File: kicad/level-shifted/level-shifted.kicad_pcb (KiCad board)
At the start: 4 copper layers, 53.5 x 76 mm, 15 parts, among them J101 PAL-1 Expansion Connector, SW101 PICO RESET, U101 74LVC245, U102 74LVC245, U103 Pico, U104 74LVC245, U105 74LVC245

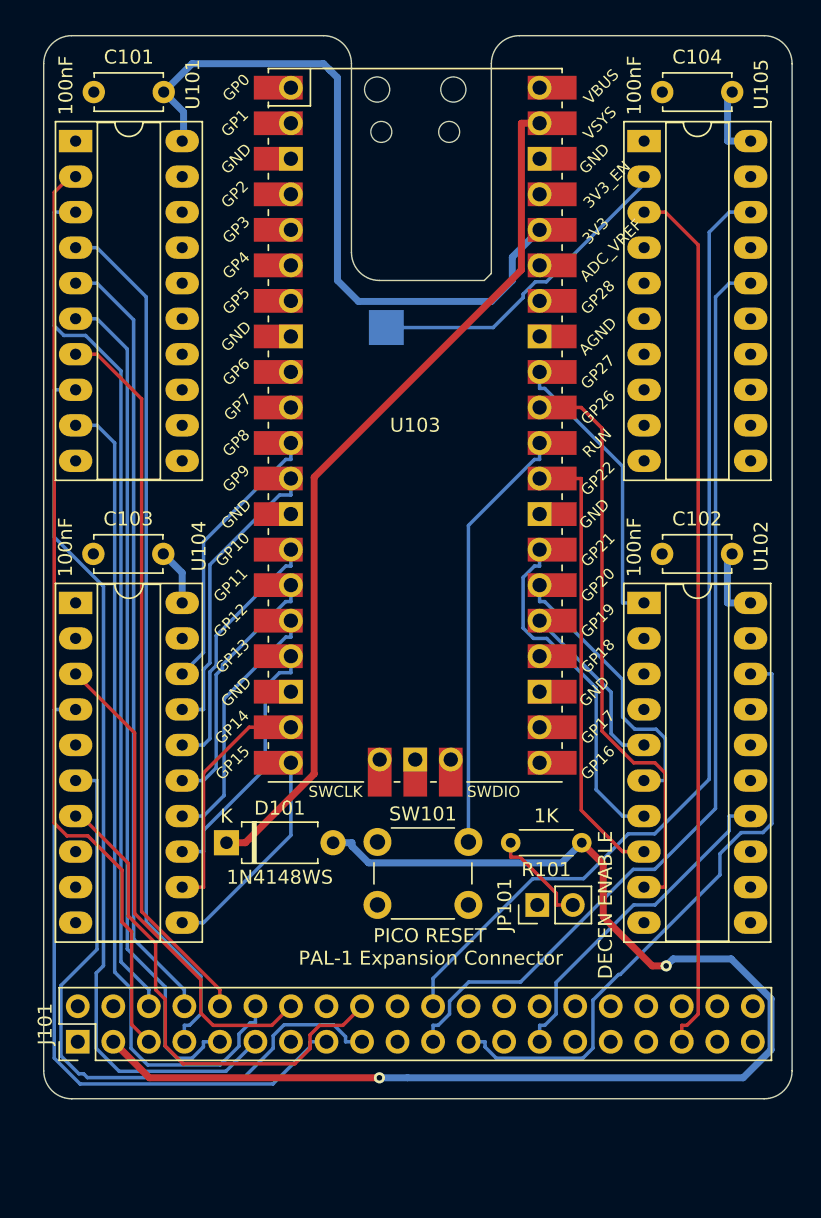
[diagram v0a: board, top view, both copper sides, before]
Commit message: Trial of multiplexed code
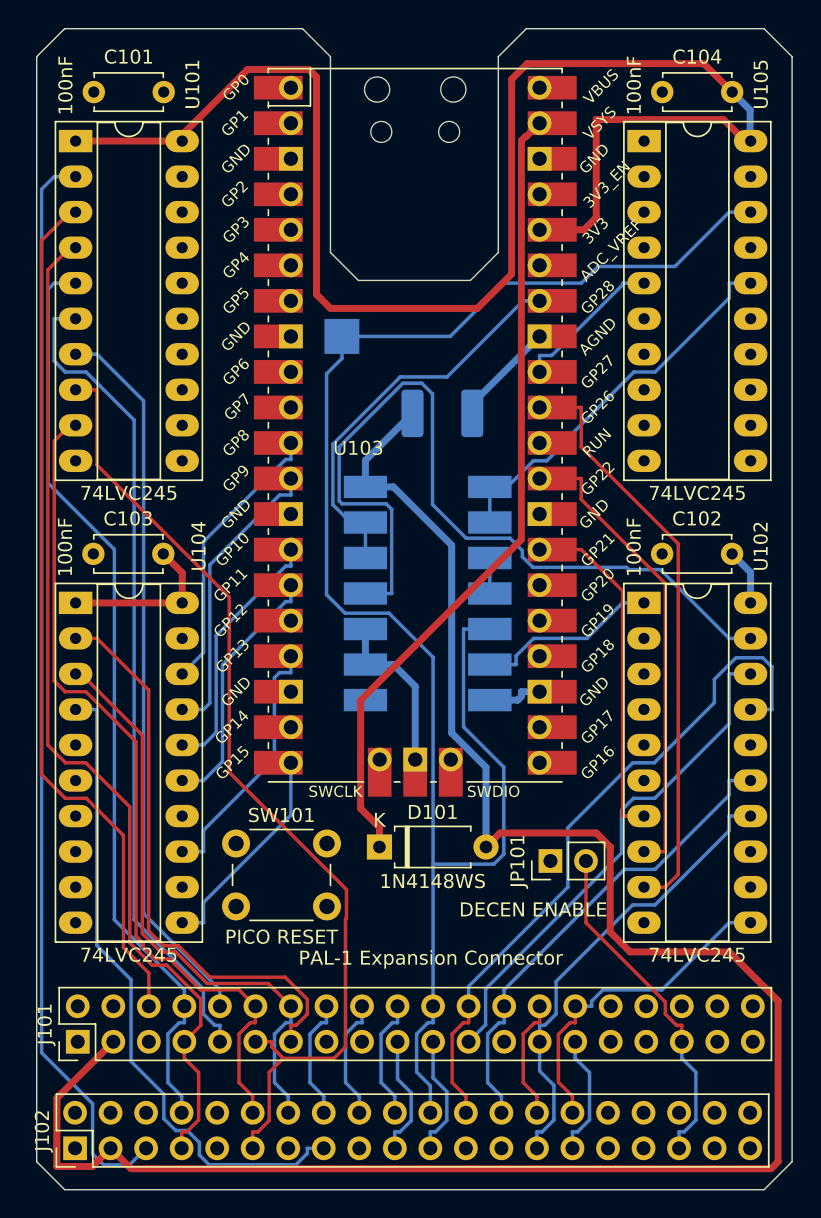
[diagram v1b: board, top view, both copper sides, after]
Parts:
- removed R101: 1K, Resistor_THT:R_Axial_DIN0204_L3.6mm_D1.6mm_P5.08mm_Horizontal
- added C105: 100nF, Capacitor_SMD:C_1812_4532Metric_Pad1.57x3.40mm_HandSolder, B.Cu at (91.0, 132.5)
- added J102: PAL-1 Expansion Connector, Connector_PinHeader_2.54mm:PinHeader_2x20_P2.54mm_Vertical, F.Cu at (64.7, 185.0)
- added U106: 74LS00, Package_DIP:DIP-14_W8.89mm_SMDSocket_LongPads, B.Cu at (89.9, 145.4)
- moved D101 10.9 mm to (86.5, 163.5)
- moved SW101 10.1 mm to (76.2, 163.2)
- moved JP101 3.28 mm to (98.7, 164.5)
- moved TP101 3.24 mm to (83.8, 127.0), turned to 90 degrees
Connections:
- JP101 pad 1: /DEN -> /~{DEN_S}
- JP101 pad 2: /~{LVDEN} -> /~{HVDEN}
- TP101 pad 1: LVPHI2 -> /HVPHI2
- U102 pad 1: /LVR~{W} -> /~{HV_W}
- U102 pad 19: GND -> /DATA_EN
- U103 pad 32: /LVR~{W} -> /~{LV_W}
- U103 pad 34: /DEN -> /~{LVDEN}
- U105 pad 1: +3.3V -> GND
- U105 pad 15: unconnected-(U105-B3-Pad15) -> /~{HV_W}
- U105 pad 2: LVPHI2 -> unconnected-(U105-A0-Pad2)
- U105 pad 3: /~{HVDEN} -> /~{DEN_S}
- U105 pad 4: /LVR~{W} -> unconnected-(U105-A2-Pad4)
- U105 pad 5: unconnected-(U105-A3-Pad5) -> /~{LV_W}
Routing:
- net /~{DEN_S}: track 0.00 -> 72.6 mm
- net /DATA_EN: track 0.00 -> 59.5 mm
- net V5: track 92.5 -> 142.0 mm, vias 2 -> 0
- net /HVPHI2: track 70.3 -> 118.9 mm
- net /DEN: track 46.3 -> 0.00 mm
- net +3.3V: track 159.7 -> 201.2 mm
- net /~{HV_W}: track 0.00 -> 38.5 mm
- net /~{HVDEN}: track 62.5 -> 24.7 mm
- net /HVR~{W}: track 67.8 -> 103.1 mm
- net /LVR~{W}: track 34.1 -> 0.00 mm
- net LVPHI2: track 23.4 -> 0.00 mm
- net GND: track 0.00 -> 22.8 mm
- net /HVA0: track 66.4 -> 86.7 mm
- net /HVA14: track 32.9 -> 50.4 mm
- net /~{LVDEN}: track 61.8 -> 44.3 mm
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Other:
- board size 53.5 x 76 mm -> 54 x 83 mm
- board text added: "WIDE BUS (VERSION 3.0)"
- board text added: "https://github.com/JeremyJStarcher/pal1-ram-rom"
- board text removed: "WIDE BUS (VERSION 2.0)"
- board text removed: "https://github.com/ JeremyJStarcher/ pal1-ram-rom"
